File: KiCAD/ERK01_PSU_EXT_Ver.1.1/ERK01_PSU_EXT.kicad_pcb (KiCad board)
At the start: 2 copper layers, 71.1 x 48.3 mm, 12 parts, among them J1 Conn_02x08_Odd_Even, J2 Conn_02x08_Odd_Even, J3 Conn_02x08_Odd_Even, J4 Conn_02x08_Odd_Even, J5 Conn_02x08_Odd_Even, J6 Conn_01x02, J7 Conn_01x03

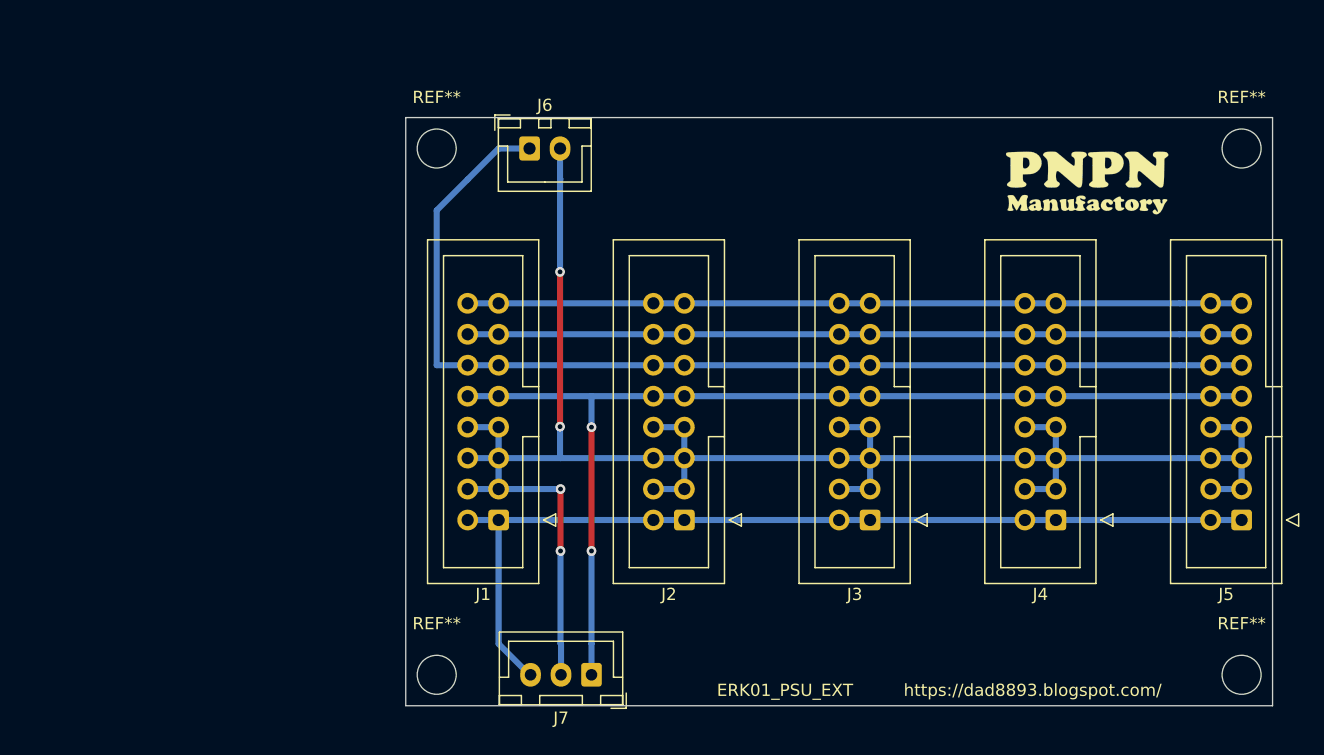
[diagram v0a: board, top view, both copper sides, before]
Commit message: Gerber
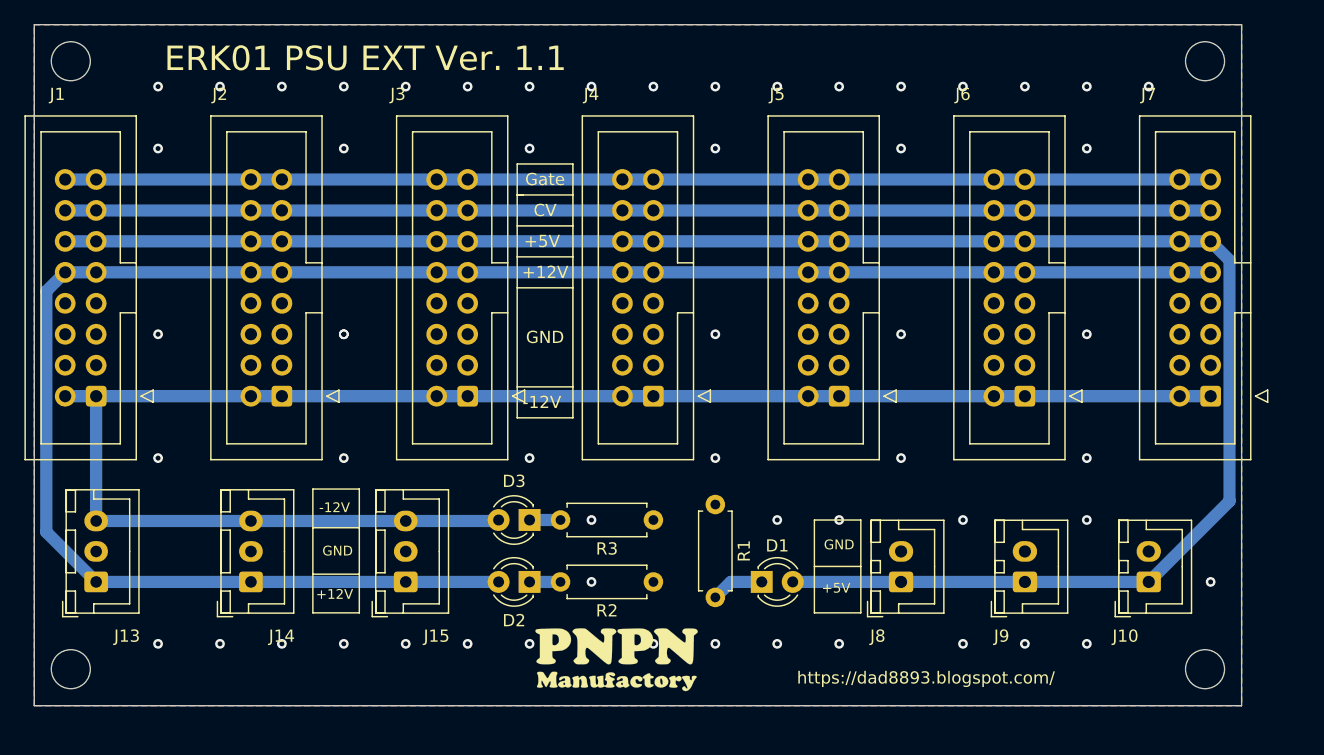
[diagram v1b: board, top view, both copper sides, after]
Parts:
- removed REF** (x4): MountingHole_3.2mm_M3, MountingHole:MountingHole_3.2mm_M3
- added D1: GREEN, LED_THT:LED_D3.0mm, F.Cu at (156.2, 116.8)
- added D2: RED, LED_THT:LED_D3.0mm, F.Cu at (137.2, 116.8)
- added D3: BLUE, LED_THT:LED_D3.0mm, F.Cu at (137.2, 111.8)
- added H1: MountingHole, MountingHole:MountingHole_3.2mm_M3, F.Cu at (99.5, 74.1)
- added H2: MountingHole, MountingHole:MountingHole_3.2mm_M3, F.Cu at (192.6, 74.1)
- added H3: MountingHole, MountingHole:MountingHole_3.2mm_M3, F.Cu at (99.5, 124.0)
- added H4: MountingHole, MountingHole:MountingHole_3.2mm_M3, F.Cu at (192.6, 124.0)
- added J10: +5V, Connector_JST:JST_XH_B2B-XH-A_1x02_P2.50mm_Vertical, F.Cu at (188.0, 116.8)
- added J13: +-12V, Connector_JST:JST_XH_B3B-XH-A_1x03_P2.50mm_Vertical, F.Cu at (101.6, 116.8)
- added J14: +-12V, Connector_JST:JST_XH_B3B-XH-A_1x03_P2.50mm_Vertical, F.Cu at (114.3, 116.8)
- added J15: +-12V, Connector_JST:JST_XH_B3B-XH-A_1x03_P2.50mm_Vertical, F.Cu at (127.0, 116.8)
- added J8: +5V, Connector_JST:JST_XH_B2B-XH-A_1x02_P2.50mm_Vertical, F.Cu at (167.6, 116.8)
- added J9: +5V, Connector_JST:JST_XH_B2B-XH-A_1x02_P2.50mm_Vertical, F.Cu at (177.8, 116.8)
- added R1: 1k, Resistor_THT:R_Axial_DIN0207_L6.3mm_D2.5mm_P7.62mm_Horizontal, F.Cu at (152.4, 110.5)
- added R2: 1k, Resistor_THT:R_Axial_DIN0207_L6.3mm_D2.5mm_P7.62mm_Horizontal, F.Cu at (147.3, 116.8)
- added R3: 1k, Resistor_THT:R_Axial_DIN0207_L6.3mm_D2.5mm_P7.62mm_Horizontal, F.Cu at (147.3, 111.8)
- J6: value Conn_01x02 -> Conn_02x08_Odd_Even; footprint Connector_JST:JST_XH_B2B-XH-A_1x02_P2.50mm_Vertical -> Connector_IDC:IDC-Header_2x08_P2.54mm_Vertical
- J7: value Conn_01x03 -> Conn_02x08_Odd_Even; footprint Connector_JST:JST_XH_B3B-XH-A_1x03_P2.50mm_Vertical -> Connector_IDC:IDC-Header_2x08_P2.54mm_Vertical
- moved J7 55.7 mm to (193.0, 101.6)
- moved G*** 55.0 mm to (144.3, 122.9)
- moved J6 45.4 mm to (177.8, 101.6), turned to 180 degrees
- moved J1 34.5 mm to (101.6, 101.6)
- moved J2 34.5 mm to (116.8, 101.6)
- moved J4 34.5 mm to (147.3, 101.6)
- moved J5 34.5 mm to (162.6, 101.6)
- moved J3 34.5 mm to (132.1, 101.6)
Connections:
- J6 pad 1: /+5V -> /-12V
- J6 pad 2: GND -> /-12V
- J7 pad 1: /+12V -> /-12V
- J7 pad 2: GND -> /-12V
- J7 pad 3: /-12V -> GND
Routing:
- net GND: track 160.2 -> 0.00 mm, vias 4 -> 57
- net /+12V: track 86.4 -> 154.7 mm, vias 2 -> 0
- net /+5V: track 88.5 -> 154.5 mm
- net /-12V: track 77.4 -> 137.3 mm
- net /Gate: track 63.5 -> 94.0 mm
- net /CV: track 63.5 -> 94.0 mm
- net Net-(D1-Pad1): track 0.00 -> 4.34 mm
- net Net-(D3-Pad1): track 0.00 -> 2.54 mm
- net Net-(D2-Pad1): track 0.00 -> 2.54 mm
- added copper zone on B.Cu, net GND
- added copper zone on F.Cu, net GND
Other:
- board size 71.1 x 48.3 mm -> 99.1 x 55.9 mm
- board text added: "+12V"
- board text added: "+5V"
- board text added: "-12V"
- board text added: "CV"
- board text added: "ERK01 PSU EXT Ver. 1.1"
- board text added: "GND"
- board text added: "Gate"
- board text removed: "ERK01_PSU_EXT"
